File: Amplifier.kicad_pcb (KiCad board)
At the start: 2 copper layers, 140 x 54 mm, 26 parts, among them J2 Input, J3 Conn_01x04, J4 output, T1 Transformer_SP_1S, U1 6N2P, U2 6P14P

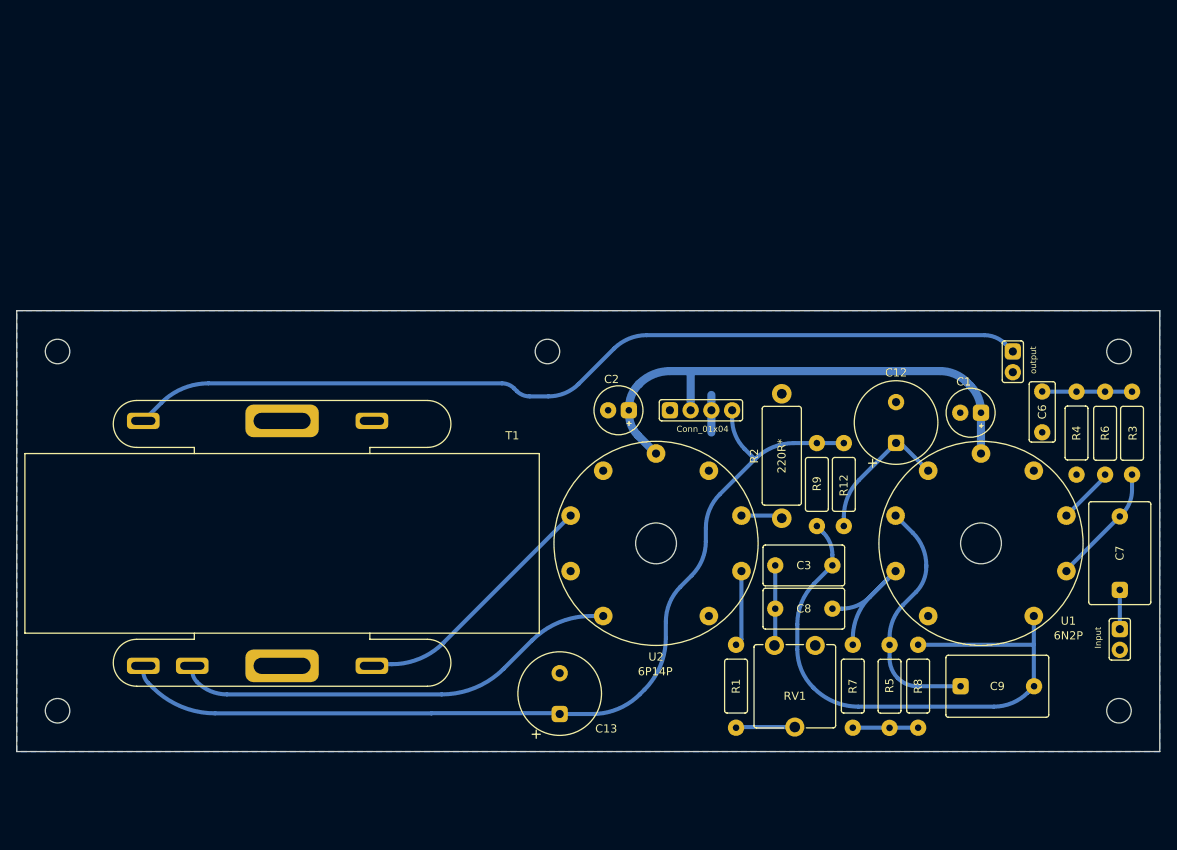
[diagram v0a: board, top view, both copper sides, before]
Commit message: New amplifier PCB
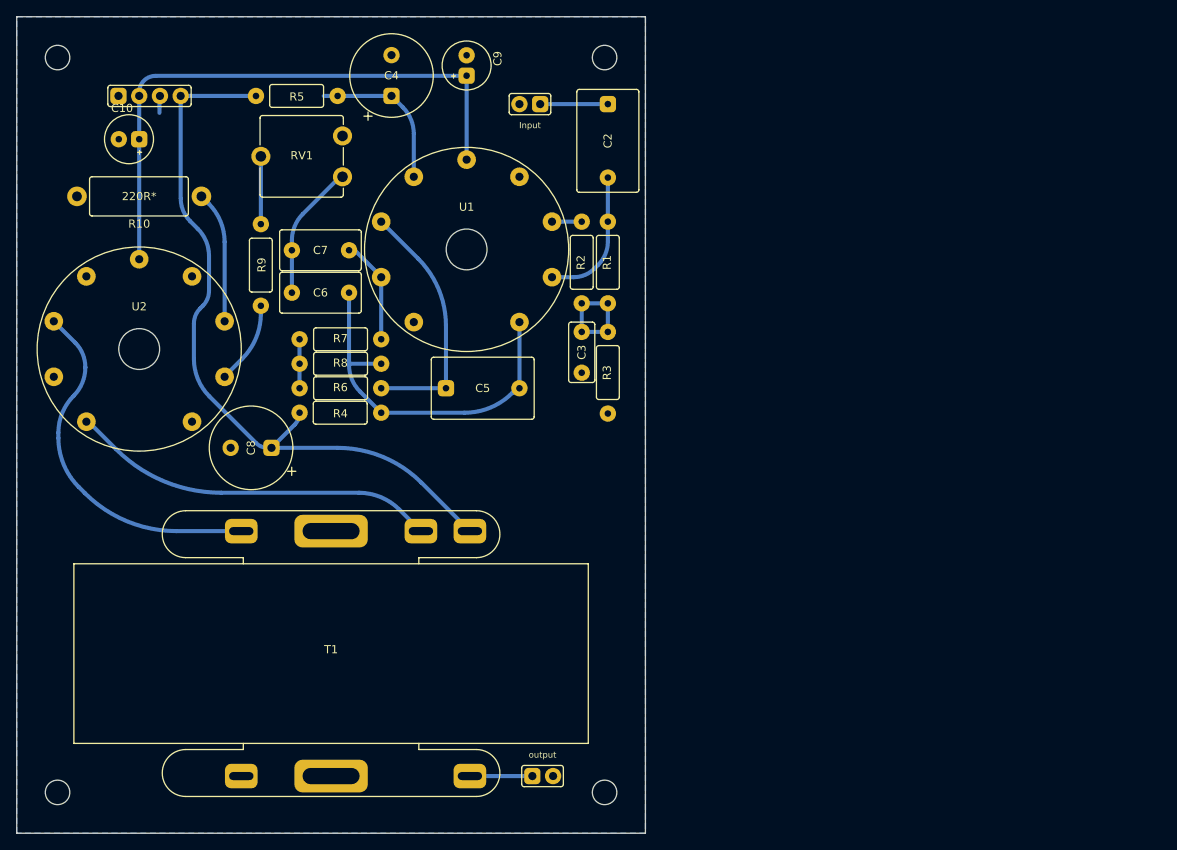
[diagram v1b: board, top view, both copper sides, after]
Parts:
- removed C1: 10uF, spdf1626_lib:C_THT_D5.0mm_P2.54mm
- removed C12, C13: 10uF, spdf1626_lib:C_THT_D10.0mm_P5.00mm
- removed J4: output, spdf1626_lib:PinHeader_1x02_P2.54mm
- removed R12: 680R, spdf1626_lib:R_THT_025W
- added C10: 10uF, spdf1626_lib:C_THT_D5.0mm_P2.5mm, F.Cu at (63.8, 55.0)
- added C4: 10uF, spdf1626_lib:C_THT_D10.0mm_P5.00mm, F.Cu at (95.9, 47.2)
- added C5: 100n, spdf1626_lib:C_THT_K73-17_P9.00mm, F.Cu at (107.1, 85.5)
- added J1: Input, spdf1626_lib:PinHeader_1x02_P2.54mm, F.Cu at (114.1, 50.7)
- added R10: 220R*, spdf1626_lib:R_THT_1W, F.Cu at (72.6, 62.0)
- C2: value 10uF -> 100n; footprint spdf1626_lib:C_THT_D5.0mm_P2.54mm -> spdf1626_lib:C_THT_K73-17_P9.00mm
- C3: value 33n opt -> 1n; footprint spdf1626_lib:C_THT_K73-17_P7.00mm -> spdf1626_lib:C_THT_K73-17_P5.00mm
- C6: value 1n -> 33n opt; footprint spdf1626_lib:C_THT_K73-17_P5.00mm -> spdf1626_lib:C_THT_K73-17_P7.00mm
- C7: value 100n -> 33n; footprint spdf1626_lib:C_THT_K73-17_P9.00mm -> spdf1626_lib:C_THT_K73-17_P7.00mm
- C8: value 33n -> 10uF; footprint spdf1626_lib:C_THT_K73-17_P7.00mm -> spdf1626_lib:C_THT_D10.0mm_P5.00mm
- C9: value 100n -> 10uF; footprint spdf1626_lib:C_THT_K73-17_P9.00mm -> spdf1626_lib:C_THT_D5.0mm_P2.5mm
- J2: value Input -> Conn_01x04; footprint spdf1626_lib:PinHeader_1x02_P2.54mm -> spdf1626_lib:PinHeader_1x04_P2.54mm
- J3: value Conn_01x04 -> output; footprint spdf1626_lib:PinHeader_1x04_P2.54mm -> spdf1626_lib:PinHeader_1x02_P2.54mm
- R1: value 6k8 -> 300k
- R2: value 220R* -> 200R; footprint spdf1626_lib:R_THT_1W -> spdf1626_lib:R_THT_025W
- R3: value 300k -> 1k8
- R4: value 1k8 -> 220k opt
- R5: value 300k -> 680R
- R6: value 200R -> 300k
- R9: value 220k opt -> 6k8
- moved J2 138.9 mm to (62.5, 49.7), turned to 90 degrees
- moved R5 106.1 mm to (84.3, 49.7), turned to 180 degrees
- moved C7 104.7 mm to (87.2, 68.6), turned to 180 degrees
- moved C9 100.0 mm to (105.1, 46.0), turned to 90 degrees
- moved R6 93.7 mm to (89.6, 85.5), turned to 0 degrees
- moved R4 90.5 mm to (89.6, 88.5), turned to 180 degrees
- moved C6 89.2 mm to (87.2, 73.8), turned to 180 degrees
- moved R8 83.6 mm to (89.6, 82.5), turned to 0 degrees
- moved RV1 81.8 mm to (89.9, 54.6), turned to 180 degrees
- moved R7 78.8 mm to (89.6, 79.5), turned to 0 degrees
- moved R9 75.2 mm to (79.9, 70.4), turned to -90 degrees
- moved U1 72.6 mm to (105.1, 68.5)
- moved C8 70.5 mm to (78.7, 92.8)
- moved U2 67.6 mm to (65.0, 80.7)
- moved R3 64.2 mm to (122.4, 83.6), turned to 90 degrees
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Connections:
- C2 pad 1: +6V -> Net-(C2-Pad1)
- C2 pad 2: GND -> Net-(C2-Pad2)
- C3 pad 2: Net-(C3-Pad2) -> GND
- C6 pad 1: Net-(C6-Pad1) -> Net-(C5-Pad2)
- C6 pad 2: GND -> Net-(C6-Pad2)
- C7 pad 2: Net-(C7-Pad2) -> Net-(C6-Pad2)
- C8 pad 1: Net-(C8-Pad1) -> 240V
- C8 pad 2: Net-(C3-Pad2) -> GND
- C9 pad 1: Net-(C9-Pad1) -> +6V
- C9 pad 2: Net-(C3-Pad1) -> GND
- J2 pad 1: Net-(C7-Pad1) -> GND
- J2 pad 2: GND -> +6V
- J3 pad 1: GND -> Left_output
- J3 pad 2: +6V -> GND
- R1 pad 1: Net-(R1-Pad1) -> Net-(C3-Pad1)
- R1 pad 2: Net-(R1-Pad2) -> Net-(C2-Pad2)
- R2 pad 1: Net-(R2-Pad1) -> Net-(C3-Pad1)
- R2 pad 2: GND -> Net-(R2-Pad2)
- R3 pad 1: Net-(C6-Pad1) -> GND
- R3 pad 2: Net-(C7-Pad2) -> Net-(C3-Pad1)
- R4 pad 1: GND -> Net-(C5-Pad2)
- R4 pad 2: Net-(C6-Pad1) -> 240V
- R5 pad 1: Net-(R5-Pad1) -> Net-(C4-Pad1)
- R5 pad 2: Net-(C9-Pad1) -> 240V
- R6 pad 1: Net-(C6-Pad1) -> Net-(R6-Pad1)
- R6 pad 2: Net-(R6-Pad2) -> Net-(C5-Pad1)
- R7 pad 1: Net-(R5-Pad1) -> Net-(R6-Pad1)
- R7 pad 2: Net-(C8-Pad1) -> Net-(C7-Pad1)
- R8 pad 1: Net-(R5-Pad1) -> Net-(R6-Pad1)
- R8 pad 2: Net-(C3-Pad1) -> Net-(C5-Pad2)
- R9 pad 1: Net-(C3-Pad1) -> Net-(R9-Pad1)
- R9 pad 2: 240V -> Net-(R9-Pad2)
- RV1 pad 1: Net-(C3-Pad2) -> GND
- RV1 pad 2: Net-(R1-Pad1) -> Net-(R9-Pad1)
- RV1 pad 3: GND -> Net-(C6-Pad2)
- U1 pad 1: Net-(C3-Pad1) -> Net-(C5-Pad2)
- U1 pad 2: Net-(C7-Pad2) -> Net-(C2-Pad2)
- U1 pad 3: Net-(R6-Pad2) -> Net-(R2-Pad2)
- U1 pad 6: Net-(C12-Pad1) -> Net-(C4-Pad1)
- U1 pad 7: Net-(C9-Pad1) -> Net-(C5-Pad1)
- U1 pad 8: Net-(C8-Pad1) -> Net-(C7-Pad1)
- U2 pad 2: Net-(R1-Pad2) -> Net-(R9-Pad2)
- U2 pad 3: Net-(R2-Pad1) -> Net-(R10-Pad1)
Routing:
- net Left_output: track 111.7 -> 7.65 mm
- net Net-(C3-Pad1): track 73.4 -> 13.4 mm
- net Net-(C5-Pad2): track 0.00 -> 45.8 mm
- net Net-(C9-Pad1): track 30.8 -> 0.00 mm
- net Net-(C5-Pad1): track 0.00 -> 30.8 mm
- net 240V: track 115.8 -> 91.6 mm
- net Net-(C8-Pad1): track 20.3 -> 0.00 mm
- net Net-(C4-Pad1): track 0.00 -> 19.1 mm
- net Net-(C12-Pad1): track 17.9 -> 0.00 mm
- net Net-(C2-Pad2): track 0.00 -> 17.1 mm
- net Net-(C6-Pad2): track 0.00 -> 16.7 mm
- net Net-(R10-Pad1): track 0.00 -> 16.2 mm
- net Net-(C7-Pad2): track 14.9 -> 0.00 mm
- net Net-(T1-Pad3): track 31.5 -> 44.5 mm
- net Net-(C6-Pad1): track 11.0 -> 0.00 mm
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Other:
- board size 140 x 54 mm -> 77 x 100 mm
